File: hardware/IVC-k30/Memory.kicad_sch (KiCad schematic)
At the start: 3 parts, among them U5 AS6C8016, U6 AS6C8016, U7 AM29F040

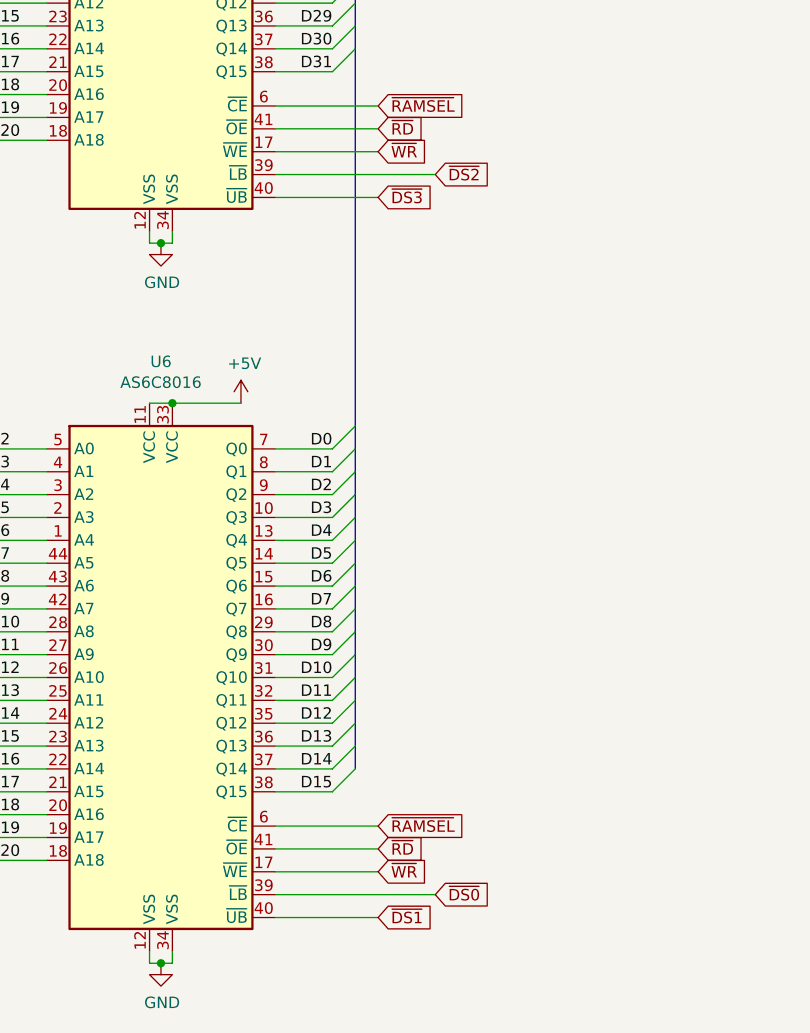
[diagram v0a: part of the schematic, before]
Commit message: Committed changes to k30 board from Oct 9th 2023
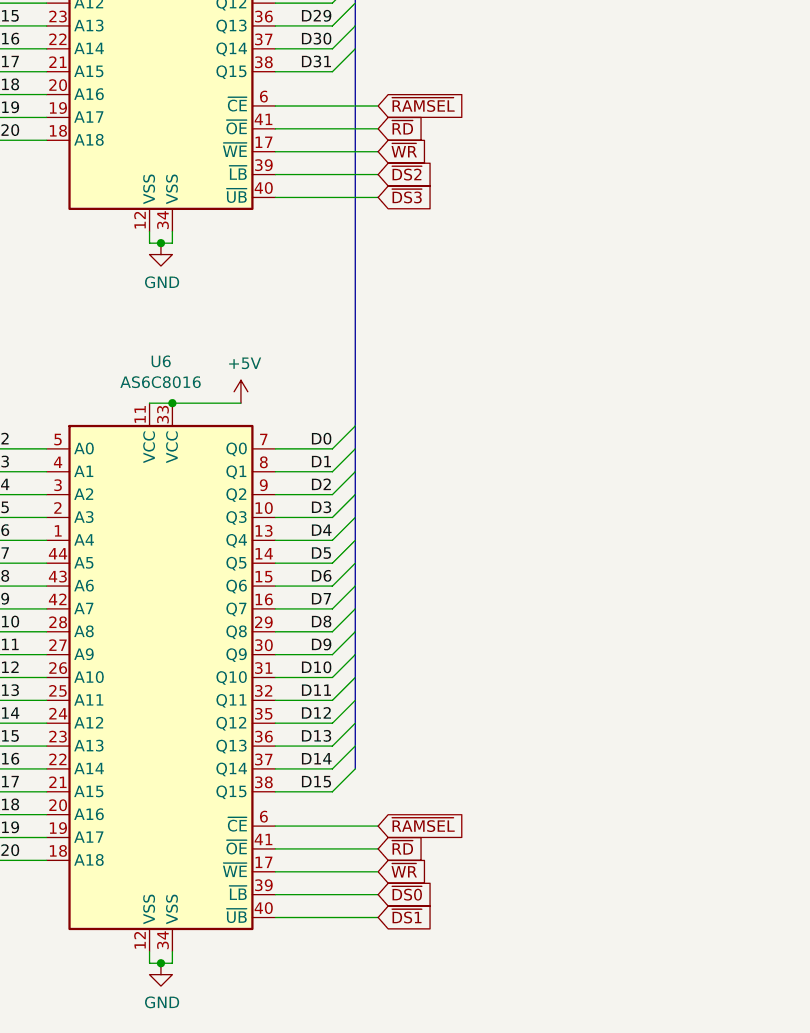
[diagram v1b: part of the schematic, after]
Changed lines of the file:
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@@
     (stroke (width 0) (type default))
   )
-  (wire (pts (xy 88.9 165.1) (xy 106.68 165.1))
+  (wire (pts (xy 88.9 165.1) (xy 100.33 165.1))
     (stroke (width 0) (type default))
   )
@@
     (stroke (width 0) (type default))
   )
-  (wire (pts (xy 88.9 85.09) (xy 106.68 85.09))
+  (wire (pts (xy 88.9 85.09) (xy 100.33 85.09))
     (stroke (width 0) (type default))
   )
@@
     )
   )
-  (global_label "~{DS2}" (shape input) (at 106.68 85.09 0) (fields_autoplaced)
+  (global_label "~{DS2}" (shape input) (at 100.33 85.09 0) (fields_autoplaced)
     (effects (font (size 1.27 1.27)) (justify left))
-    (property "Intersheetrefs" "${INTERSHEET_REFS}" (at 0 0 0)
+    (property "Intersheetrefs" "${INTERSHEET_REFS}" (at -6.35 0 0)
       (effects (font (size 1.27 1.27)) hide)
     )
@@
     )
   )
-  (global_label "~{DS0}" (shape input) (at 106.68 165.1 0) (fields_autoplaced)
+  (global_label "~{DS0}" (shape input) (at 100.33 165.1 0) (fields_autoplaced)
     (effects (font (size 1.27 1.27)) (justify left))
-    (property "Intersheetrefs" "${INTERSHEET_REFS}" (at 0 0 0)
+    (property "Intersheetrefs" "${INTERSHEET_REFS}" (at -6.35 0 0)
       (effects (font (size 1.27 1.27)) hide)
     )
